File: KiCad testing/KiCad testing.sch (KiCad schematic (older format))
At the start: 4 parts

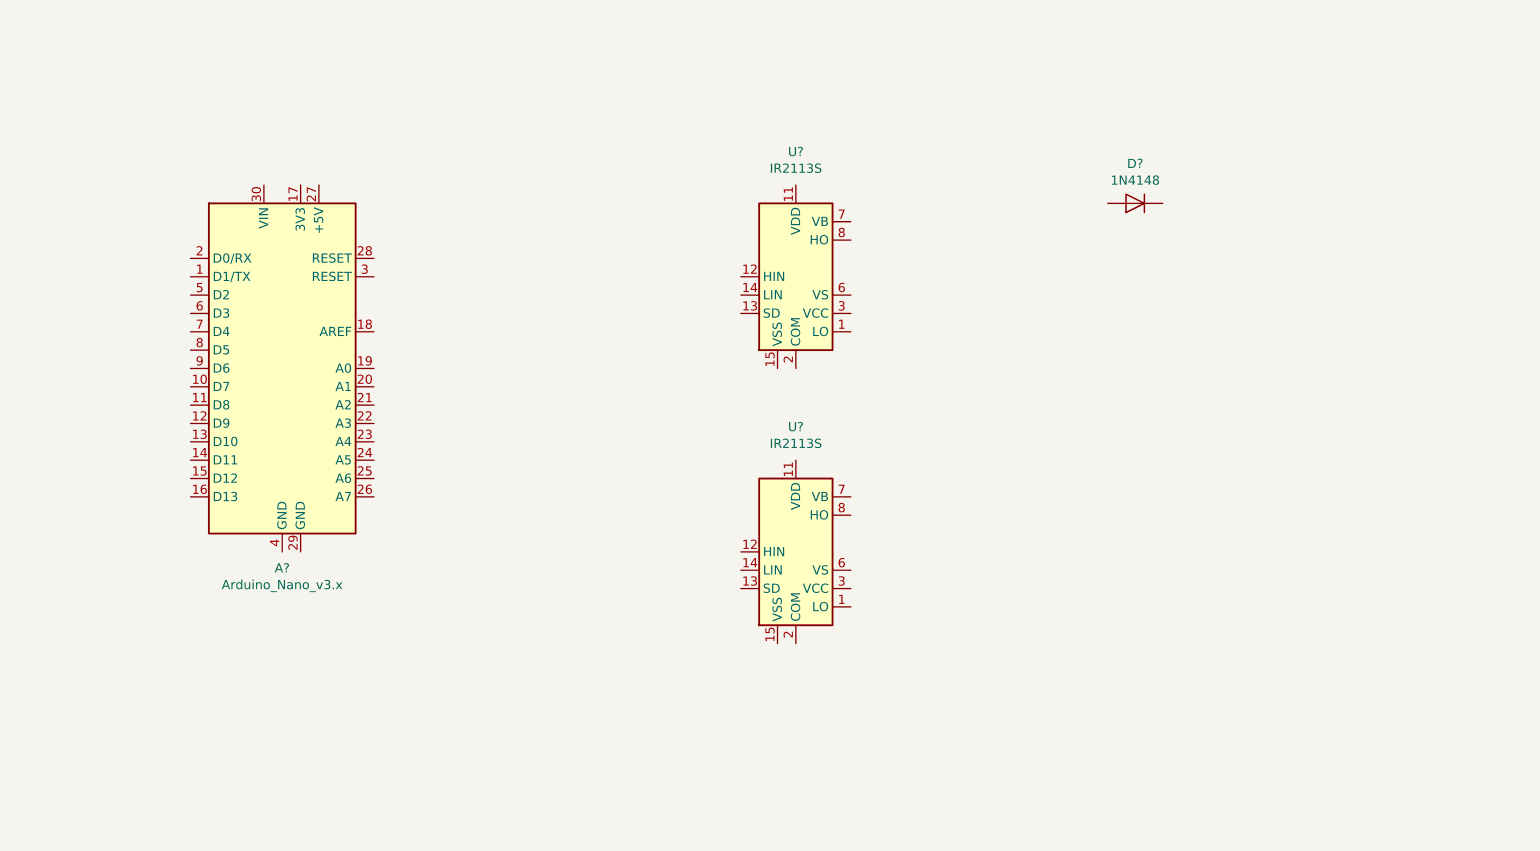
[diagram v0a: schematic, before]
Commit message: KiCad Schematics
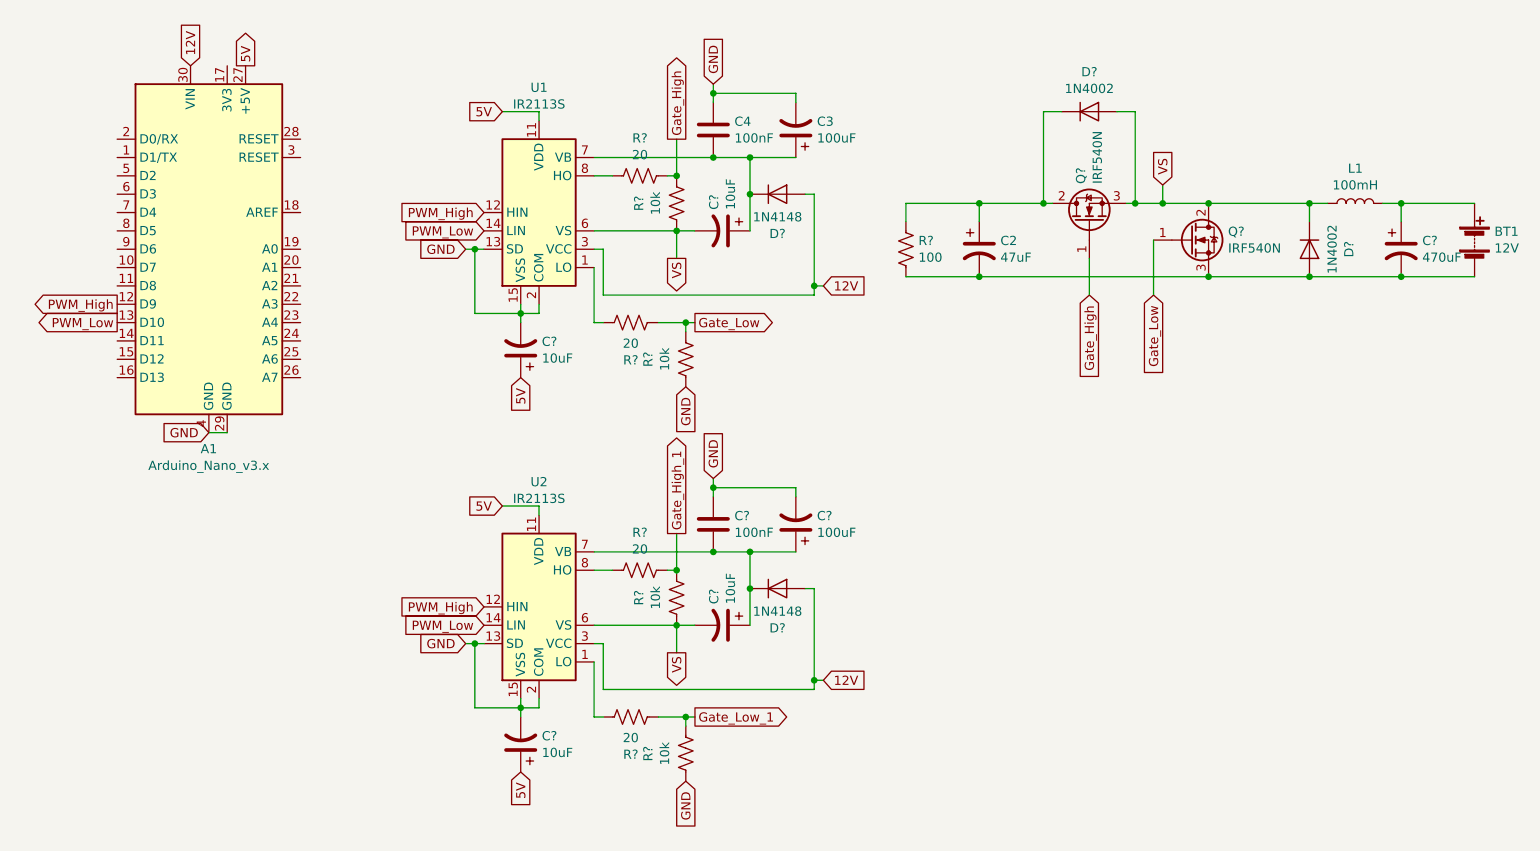
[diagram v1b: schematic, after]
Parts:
- removed U?: IR2113S, Package_SO:SOIC-16W_7.5x10.3mm_P1.27mm, symbol Driver_FET:IR2113S
- added BT1: 12V, symbol Device:Battery
- added C2: 47uF, symbol Device:CP1
- added C3, C?: 100uF, symbol Device:CP1
- added C4, C?: 100nF, symbol Device:C
- added C? (x4): 10uF, symbol Device:CP1
- added C?: 470uF, symbol Device:CP1
- added D?: 1N4148, Diode_THT:D_DO-35_SOD27_P7.62mm_Horizontal, symbol Diode:1N4148
- added D? (x2): 1N4002, Diode_THT:D_DO-41_SOD81_P10.16mm_Horizontal, symbol Diode:1N4002
- added L1: 100mH, symbol Device:L
- added Q? (x2): IRF540N, Package_TO_SOT_THT:TO-220-3_Vertical, symbol Transistor_FET:IRF540N
- added R? (x4): 20, symbol Device:R_US
- added R? (x4): 10k, symbol Device:R_US
- added R?: 100, symbol Device:R_US
- added U2: IR2113S, Package_SO:SOIC-16W_7.5x10.3mm_P1.27mm, symbol Driver_FET:IR2113S
- gave numbers to parts that had none: 2
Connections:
- net PWM_High: now reaches A1.12 (D9)
- net PWM_High: now also U1.12 (HIN), U2.12 (HIN)
- net PWM_Low: now reaches A1.13 (D10)
- net PWM_Low: now also U1.14 (LIN), U2.14 (LIN)
- net 5V: now reaches A1.27 (+5V)
- net 5V: now also U1.11 (VDD), C?.1, C?.1, U2.11 (VDD)
- net GND: now reaches A1.29 (GND)
- net GND: now also A1.4 (GND), U1.13 (SD), U1.15 (VSS), U1.2 (COM), C3.2, C4.1, C?.1, C?.2, C?.2, C?.2, R?.1, R?.1, U2.13 (SD), U2.15 (VSS), U2.2 (COM)
- net 12V: now reaches A1.30 (VIN)
- net 12V: now also D?.2 (A), U1.3 (VCC), D?.2 (A), U2.3 (VCC)
- net at U1.1 (LO): now also R?.2
- net VS: now reaches U1.6 (VS)
- net VS: now also C?.2, C?.2, D?.1 (K), D?.2 (A), L1.1, Q?.2 (D), Q?.3 (S), R?.1, R?.1, U2.6 (VS)
- net at U1.7 (VB): now also D?.1 (K), C3.1, C4.2, C?.1
- net at U1.8 (HO): now also R?.1
- new net: R?.2, U2.1 (LO)
- new net: C?.1, C?.1, C?.2, D?.1 (K), U2.7 (VB)
- new net: R?.1, U2.8 (HO)
- new net: C2.1, D?.1 (K), Q?.2 (D), R?.1
- new net: BT1.2 (-), C2.2, C?.2, D?.2 (A), Q?.3 (S), R?.2
- new net: BT1.1 (+), C?.1, L1.2
- new net Gate_High: Q?.1 (G), R?.2, R?.2
- new net Gate_High_1: R?.2, R?.2
- new net Gate_Low: Q?.1 (G), R?.1, R?.2
- new net Gate_Low_1: R?.1, R?.2
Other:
- moved on the sheet: A1, D?, U1
